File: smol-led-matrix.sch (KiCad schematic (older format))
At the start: 76 parts, among them J2 TagConnect_TC2030_SWD, SW1 SW_Push, SW2 SW_Push, U1 STM32L433CBTx

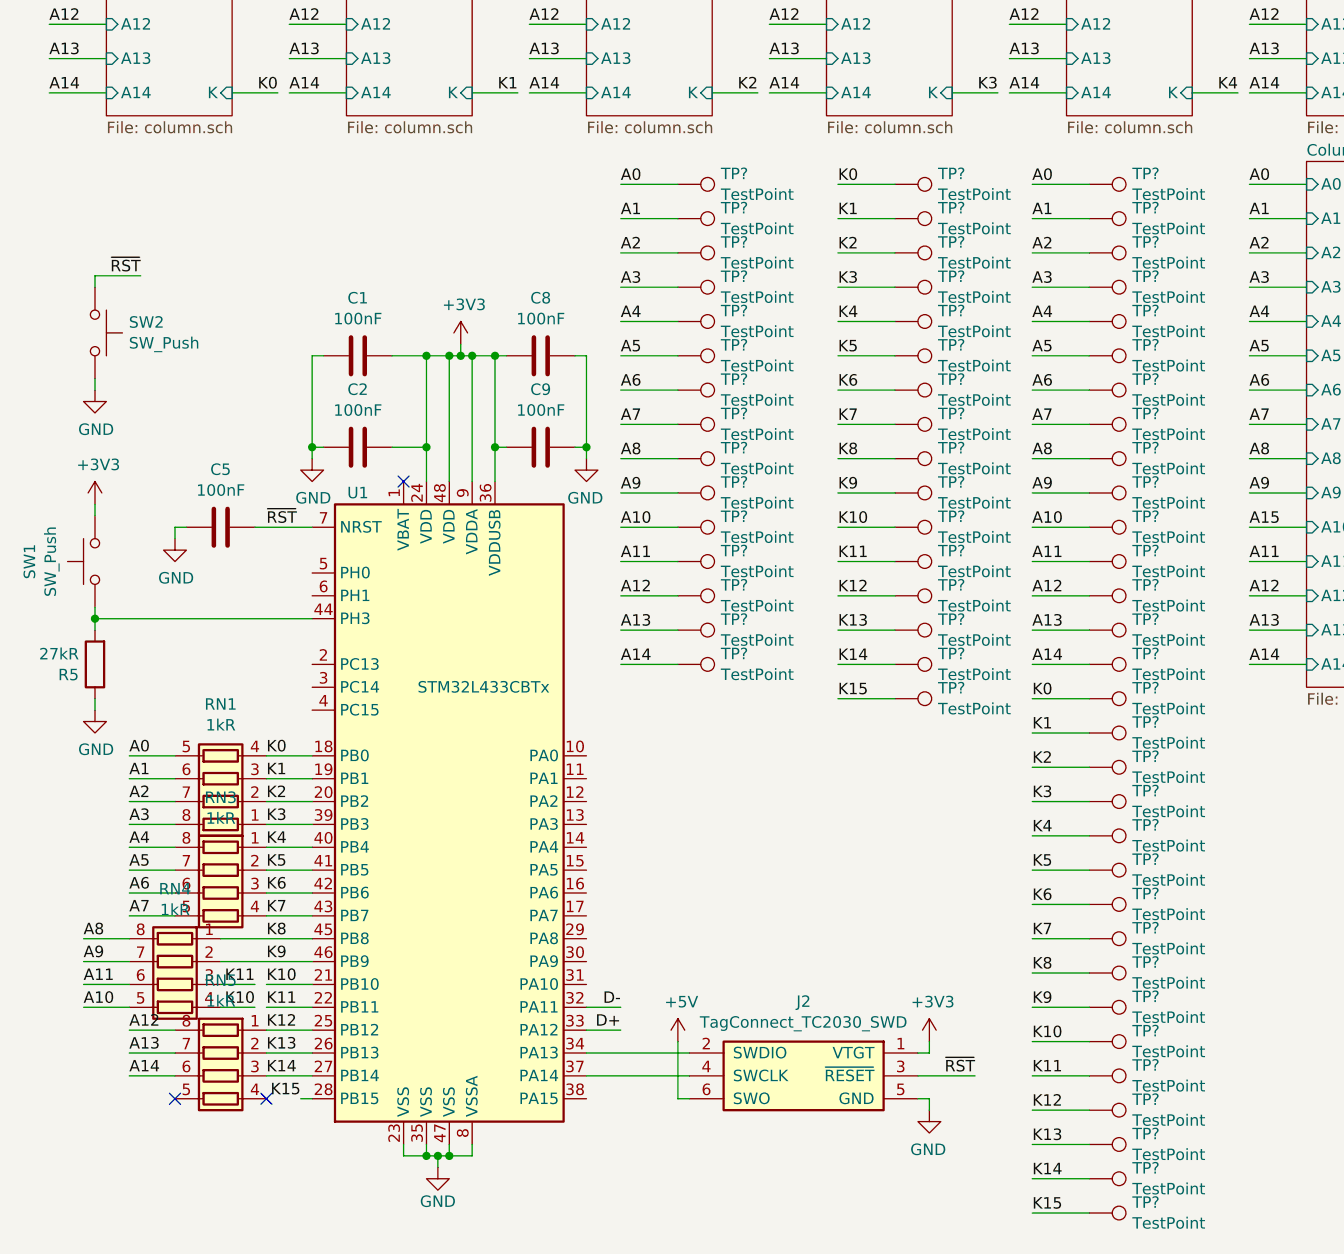
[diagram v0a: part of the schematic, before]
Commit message: Layout half done
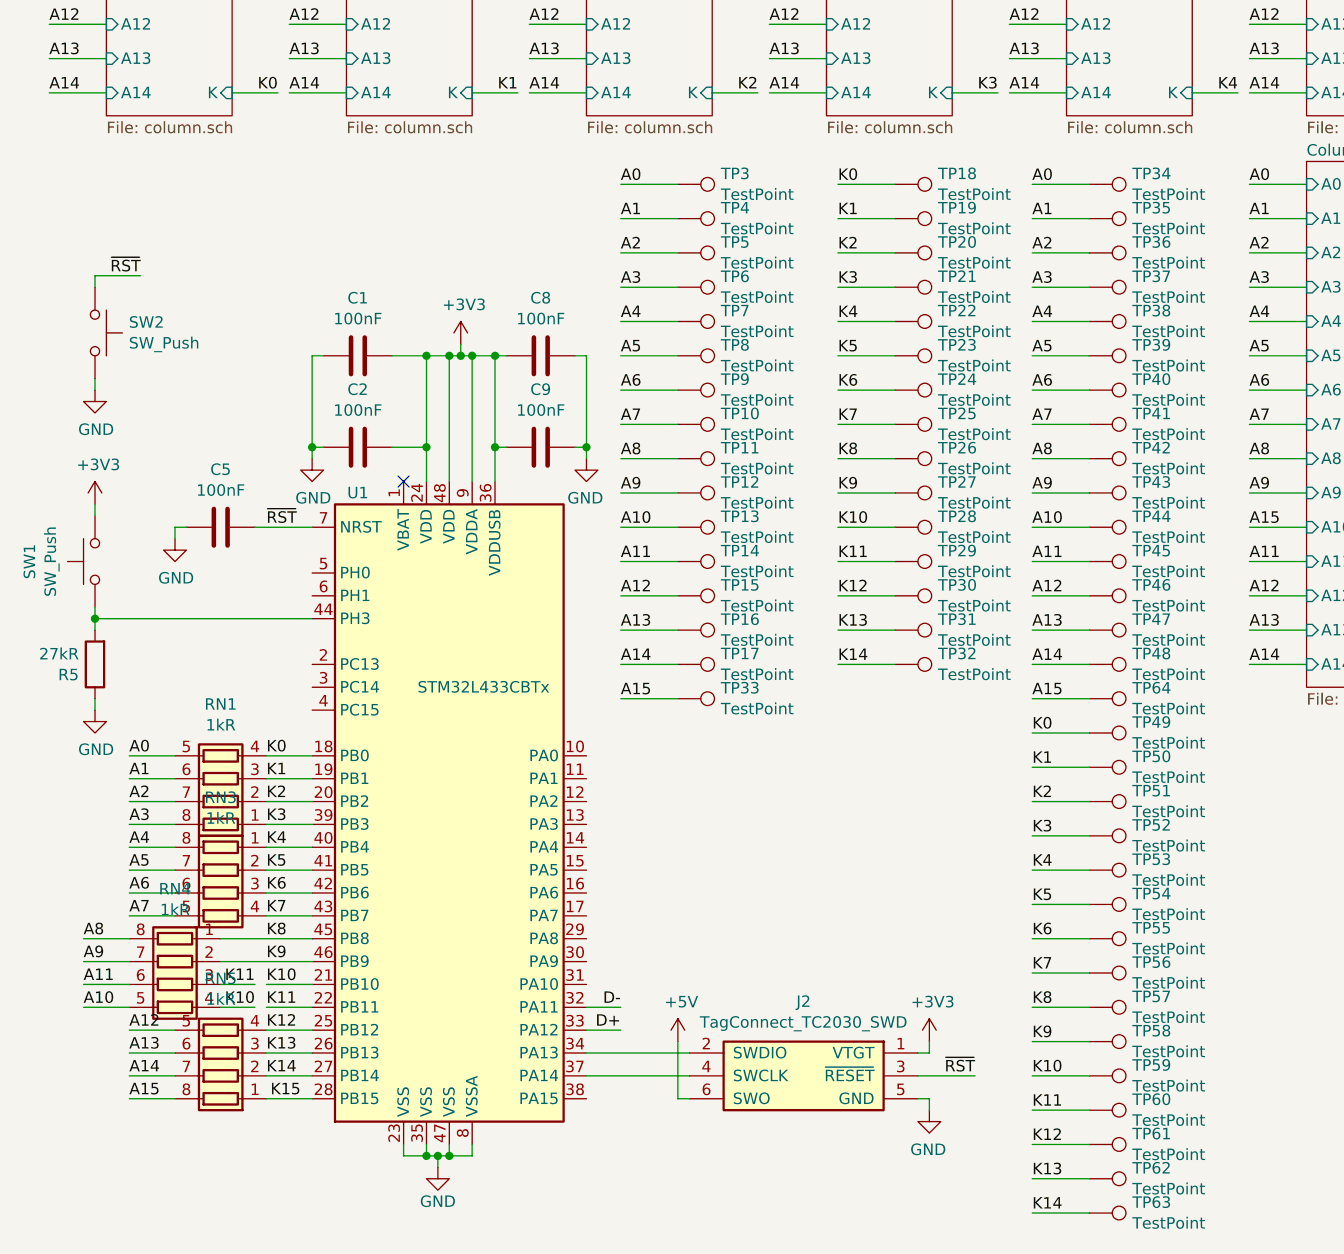
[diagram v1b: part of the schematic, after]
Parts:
- gave numbers to parts that had none: 62
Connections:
- net A12: now also RN5.5 (R4.2); no longer RN5.8 (R1.2)
- net A13: now also RN5.6 (R3.2); no longer RN5.7 (R2.2)
- net A14: now also RN5.7 (R2.2); no longer RN5.6 (R3.2)
- net A15: now also RN5.8 (R1.2), TP33.1, TP64.1
- net K12: now also RN5.4 (R4.1); no longer RN5.1 (R1.1)
- net K13: now also RN5.3 (R3.1); no longer RN5.2 (R2.1)
- net K14: now also RN5.2 (R2.1); no longer RN5.3 (R3.1)
- net K15: now also RN5.1 (R1.1); no longer TP33.1, TP64.1
- no-connect marks 3 -> 1
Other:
- moved on the sheet: TP33, TP49, TP50, TP51, TP52, TP53, TP54, TP55, TP56, TP57, TP58, TP59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
